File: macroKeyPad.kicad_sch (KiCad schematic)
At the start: 17 parts, among them U1 kb2040

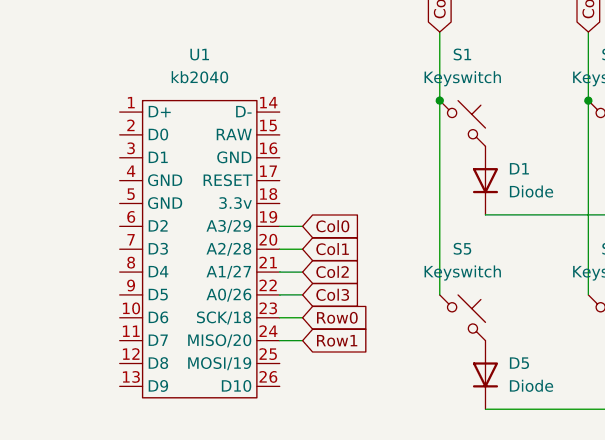
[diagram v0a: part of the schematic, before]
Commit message: pretty close to being done
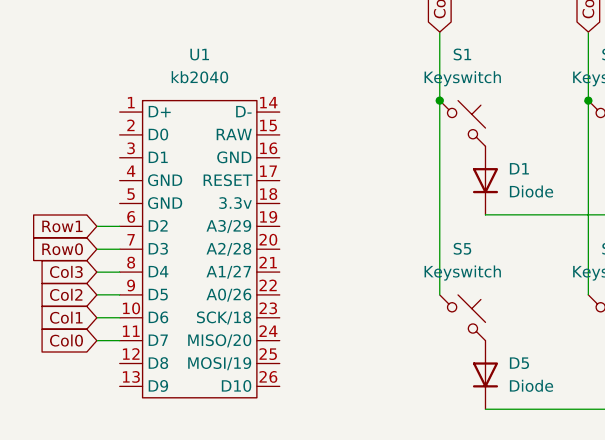
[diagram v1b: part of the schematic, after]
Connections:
- net Col0: now also U1.11 (D7); no longer U1.19 (A3/29)
- net Col1: now also U1.10 (D6); no longer U1.20 (A2/28)
- net Col2: now also U1.9 (D5); no longer U1.21 (A1/27)
- net Col3: now also U1.8 (D4); no longer U1.22 (A0/26)
- net Row0: now also U1.7 (D3); no longer U1.23 (SCK/18)
- net Row1: now also U1.6 (D2); no longer U1.24 (MISO/20)

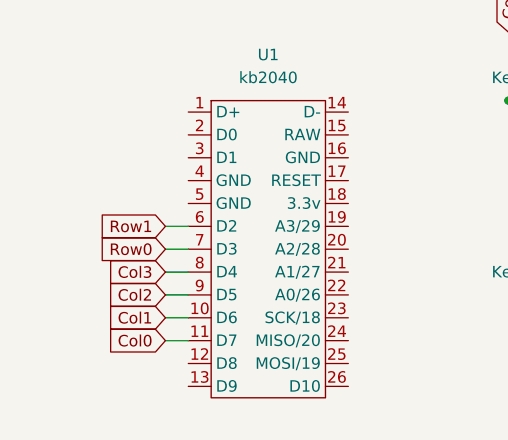
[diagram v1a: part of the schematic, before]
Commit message: wiring
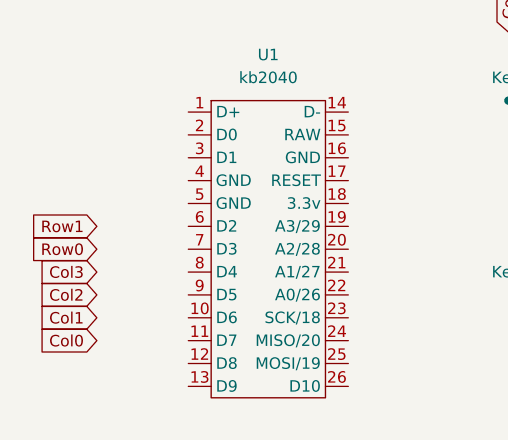
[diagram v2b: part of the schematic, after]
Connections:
- net Col0: no longer U1.11 (D7)
- net Col1: no longer U1.10 (D6)
- net Col2: no longer U1.9 (D5)
- net Col3: no longer U1.8 (D4)
- net Row0: no longer U1.7 (D3)
- net Row1: no longer U1.6 (D2)
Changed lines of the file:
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@@
-	(wire
-		(pts
-			(xy 59.69 74.93) (xy 57.15 74.93)
-		)
-		(stroke
-			(width 0)
-			(type default)
-		)
-	)
-	(wire
-		(pts
-			(xy 59.69 67.31) (xy 57.15 67.31)
-		)
-		(stroke
-			(width 0)
-			(type default)
-		)
-	)
-	(wire
-		(pts
-			(xy 59.69 69.85) (xy 57.15 69.85)
-		)
-		(stroke
-			(width 0)
-			(type default)
-		)
-	)
-	(wire
-		(pts
-			(xy 59.69 77.47) (xy 57.15 77.47)
-		)
-		(stroke
-			(width 0)
-			(type default)
-		)
-	)
 	(wire
 		(pts
@@
 	(wire
 		(pts
-			(xy 59.69 64.77) (xy 57.15 64.77)
-		)
-		(stroke
-			(width 0)
-			(type default)
-		)
-	)
-	(wire
-		(pts
 			(xy 149.86 85.09) (xy 160.02 85.09)
 		)
@@
 	(wire
 		(pts
-			(xy 59.69 72.39) (xy 57.15 72.39)
-		)
-		(stroke
-			(width 0)
-			(type default)
-		)
-	)
-	(wire
-		(pts
 			(xy 133.35 63.5) (xy 149.86 63.5)
 		)
@@
 	(global_label "Col3"
 		(shape input)
-		(at 57.15 69.85 180)
-		(fields_autoplaced yes)
-		(effects
-			(font
-				(size 1.27 1.27)
-			)
-			(justify right)
-		)
-		(property "Intersheetrefs" "${INTERSHEET_REFS}"
-			(at 49.8711 69.85 0)
+		(at 49.53 69.85 180)
+		(fields_autoplaced yes)
+		(effects
+			(font
+				(size 1.27 1.27)
+			)
+			(justify right)
+		)
+		(property "Intersheetrefs" "${INTERSHEET_REFS}"
+			(at 42.2511 69.85 0)
 			(effects
 				(font
@@
 	(global_label "Col0"
 		(shape input)
-		(at 57.15 77.47 180)
-		(fields_autoplaced yes)
-		(effects
-			(font
-				(size 1.27 1.27)
-			)
-			(justify right)
-		)
-		(property "Intersheetrefs" "${INTERSHEET_REFS}"
-			(at 49.8711 77.47 0)
+		(at 49.53 77.47 180)
+		(fields_autoplaced yes)
+		(effects
+			(font
+				(size 1.27 1.27)
+			)
+			(justify right)
+		)
+		(property "Intersheetrefs" "${INTERSHEET_REFS}"
+			(at 42.2511 77.47 0)
 			(effects
 				(font
@@
 	(global_label "Row1"
 		(shape input)
-		(at 57.15 64.77 180)
-		(fields_autoplaced yes)
-		(effects
-			(font
-				(size 1.27 1.27)
-			)
-			(justify right)
-		)
-		(property "Intersheetrefs" "${INTERSHEET_REFS}"
-			(at 49.2058 64.77 0)
+		(at 49.53 64.77 180)
+		(fields_autoplaced yes)
+		(effects
+			(font
+				(size 1.27 1.27)
+			)
+			(justify right)
+		)
+		(property "Intersheetrefs" "${INTERSHEET_REFS}"
+			(at 41.5858 64.77 0)
 			(effects
 				(font
@@
 	(global_label "Col1"
 		(shape input)
-		(at 57.15 74.93 180)
-		(fields_autoplaced yes)
-		(effects
-			(font
-				(size 1.27 1.27)
-			)
-			(justify right)
-		)
-		(property "Intersheetrefs" "${INTERSHEET_REFS}"
-			(at 49.8711 74.93 0)
+		(at 49.53 74.93 180)
+		(fields_autoplaced yes)
+		(effects
+			(font
+				(size 1.27 1.27)
+			)
+			(justify right)
+		)
+		(property "Intersheetrefs" "${INTERSHEET_REFS}"
+			(at 42.2511 74.93 0)
 			(effects
 				(font
@@
 	(global_label "Col2"
 		(shape input)
-		(at 57.15 72.39 180)
-		(fields_autoplaced yes)
-		(effects
-			(font
-				(size 1.27 1.27)
-			)
-			(justify right)
-		)
-		(property "Intersheetrefs" "${INTERSHEET_REFS}"
-			(at 49.8711 72.39 0)
+		(at 49.53 72.39 180)
+		(fields_autoplaced yes)
+		(effects
+			(font
+				(size 1.27 1.27)
+			)
+			(justify right)
+		)
+		(property "Intersheetrefs" "${INTERSHEET_REFS}"
+			(at 42.2511 72.39 0)
 			(effects
 				(font
@@
 	(global_label "Row0"
 		(shape input)
-		(at 57.15 67.31 180)
-		(fields_autoplaced yes)
-		(effects
-			(font
-				(size 1.27 1.27)
-			)
-			(justify right)
-		)
-		(property "Intersheetrefs" "${INTERSHEET_REFS}"
-			(at 49.2058 67.31 0)
-			(effects
-				(font
+		(at 49.53 67.31 180)
+		(fields_autoplaced yes)
+		(effects
+			(font
+				(size 1.27 1.27)
+			)
+			(justify right)
+		)
+		(property "Intersheetrefs" "${INTERSHEET_REFS}"
+			(at 41.5858 67.31 0)
+			(effects
+				(font
